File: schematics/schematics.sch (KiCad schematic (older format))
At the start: 5 parts

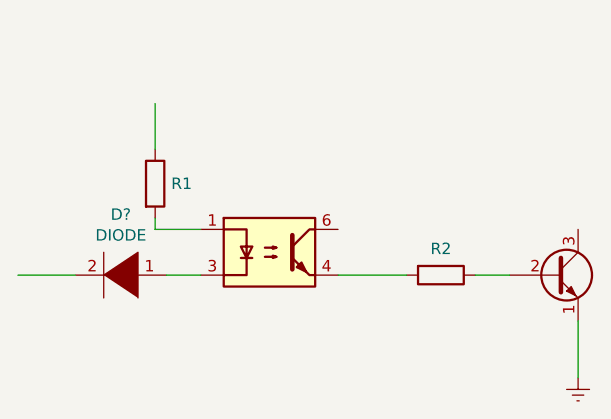
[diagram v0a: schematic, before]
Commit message: Edit the base of the circuit
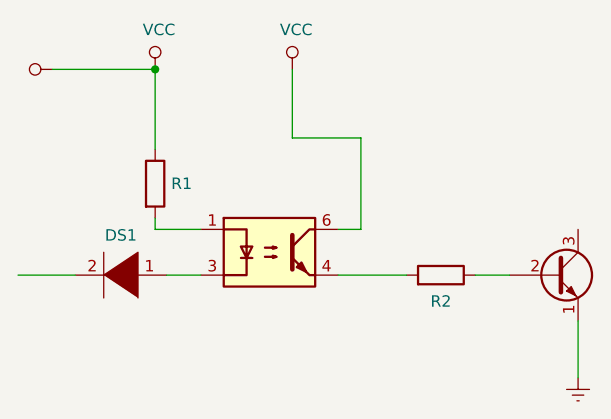
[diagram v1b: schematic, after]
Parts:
- D?: value DIODE -> DS1
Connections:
- net labels added: VCC
- wire segments 8 -> 13
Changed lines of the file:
@@
 EESchema Schematic File Version 4
+LIBS:schematics-cache
 EELAYER 29 0
 EELAYER END
@@
 U 1 1 5C8C1EFD
 P 4550 4700
-F 0 "D?" H 4550 4435 50  0000 C CNN
-F 1 "DIODE" H 4550 4526 50  0000 C CNN
+F 0 "D?" H 4550 4435 50  0001 C CNN
+F 1 "DS1" H 4550 4526 50  0000 C CNN
 F 2 "" H 4550 4700 50  0001 C CNN
 F 3 "~" H 4550 4700 50  0001 C CNN
@@
 Wire Wire Line
 	4350 4700 4100 4700
-Wire Wire Line
-	4700 4150 4700 3950
 Wire Wire Line
 	5500 4700 5800 4700
@@
 F 3 "~" H 5950 4700 50  0001 C CNN
 	1    5950 4700
-	0    1    1    0
+	0    1    -1   0
 $EndComp
 Wire Wire Line
@@
 	1    0    0    -1
 $EndComp
+$Comp
+L power:VCC #PWR?
+U 1 1 5C8BCB84
+P 4700 3800
+F 0 "#PWR?" H 4700 3650 50  0001 C CNN
+F 1 "VCC" H 4717 3973 50  0000 C CNN
+F 2 "" H 4700 3800 50  0001 C CNN
+F 3 "" H 4700 3800 50  0001 C CNN
+	1    4700 3800
+	1    0    0    -1
+$EndComp
+Wire Wire Line
+	4700 3800 4250 3800
+Connection ~ 4700 3800
+$Comp
+L power:VCC #PWR?
+U 1 1 5C8BE04C
+P 4250 3800
+F 0 "#PWR?" H 4250 3650 50  0001 C CNN
+F 1 "VCC" V 4268 3927 50  0001 L CNN
+F 2 "" H 4250 3800 50  0001 C CNN
+F 3 "" H 4250 3800 50  0001 C CNN
+	1    4250 3800
+	0    -1   -1   0
+$EndComp
+Wire Wire Line
+	4700 3800 4700 4150
+Wire Wire Line
+	5500 4500 5600 4500
+Wire Wire Line
+	5600 4500 5600 4100
+Wire Wire Line
+	5600 4100 5300 4100
+Wire Wire Line
+	5300 4100 5300 3800
+$Comp
+L power:VCC #PWR?
+U 1 1 5C8C0019
+P 5300 3800
+F 0 "#PWR?" H 5300 3650 50  0001 C CNN
+F 1 "VCC" H 5317 3973 50  0000 C CNN
+F 2 "" H 5300 3800 50  0001 C CNN
+F 3 "" H 5300 3800 50  0001 C CNN
+	1    5300 3800
+	1    0    0    -1
+$EndComp
